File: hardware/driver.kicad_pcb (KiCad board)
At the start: 2 copper layers, 24 x 23 mm, 15 parts, among them Q1 BSS84, Q2 BSS138, Q3 BSS138, Q4 BSS84, Q5 BSS138, Q6 BSS138

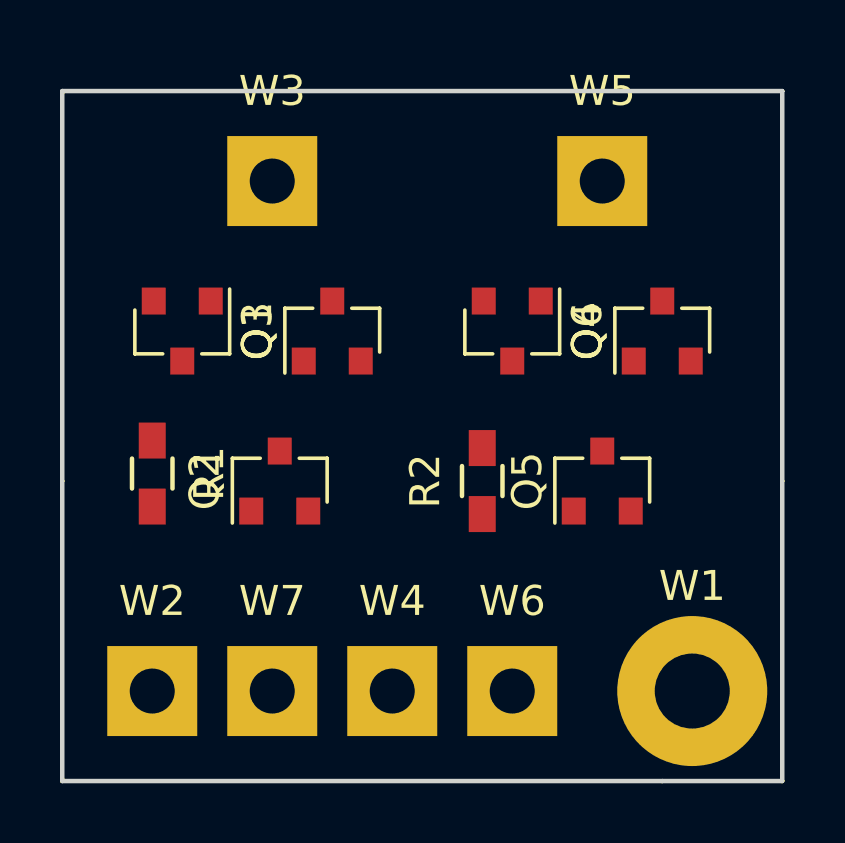
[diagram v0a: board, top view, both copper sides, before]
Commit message: Routing
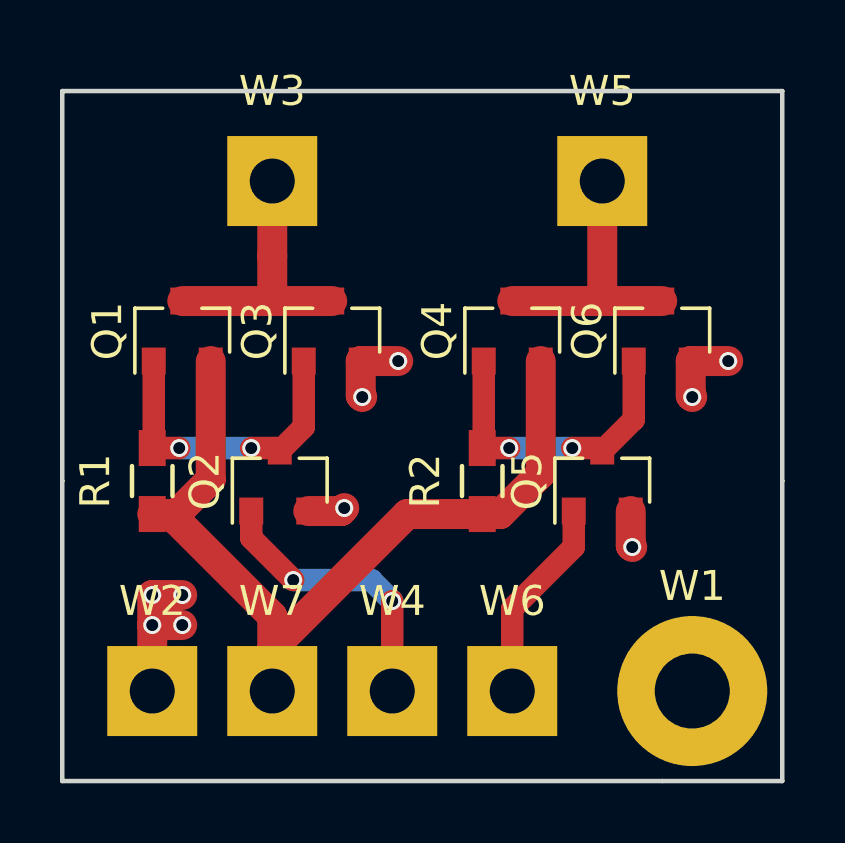
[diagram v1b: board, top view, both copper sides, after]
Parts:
- moved R1 0.25 mm to (103.0, 70.0), turned to 90 degrees
- turned Q1 to 90 degrees
- turned Q4 to 90 degrees
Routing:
- net VCC: track 0.00 -> 30.1 mm
- net GND: track 0.00 -> 12.6 mm, vias 0 -> 10
- net Net-(Q1-Pad1): track 0.00 -> 10.7 mm, vias 0 -> 2
- net Net-(Q4-Pad1): track 0.00 -> 10.4 mm, vias 0 -> 2
- net Net-(Q2-Pad1): track 0.00 -> 9.47 mm, vias 0 -> 2
- net Net-(Q4-Pad3): track 0.00 -> 9.04 mm
- net Net-(Q1-Pad3): track 0.00 -> 9.00 mm
- net Net-(Q5-Pad1): track 0.00 -> 6.85 mm
- added copper zone on B.Cu, net GND
